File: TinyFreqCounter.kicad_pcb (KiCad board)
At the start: 2 copper layers, 99.1 x 82.5 mm, 30 parts, among them J1 Conn_01x20_Socket, J2 Conn_01x20_Socket, J3 Barrel_Jack_Switch, J4 Conn_01x06_Pin, J5 Conn_01x08_Pin, J6 Conn_01x06_Pin, J7 Conn_01x02_Pin, SW1 SW_SPDT, SW2 SW_SPST, U2 HM678127_SOJ32_Arranged, U3 PIC18F57Q43-IPT

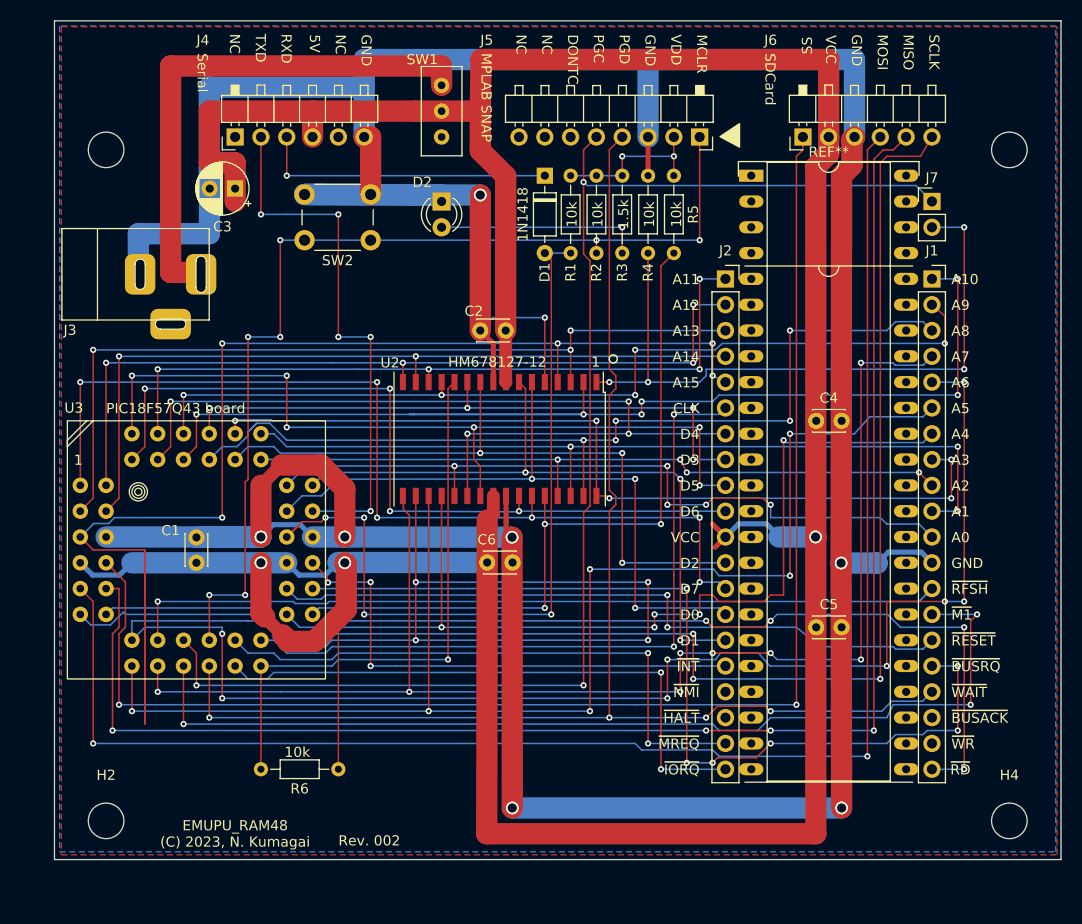
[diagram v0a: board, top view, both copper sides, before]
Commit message: Rev001: garber generated, and ordered to JLCPCB
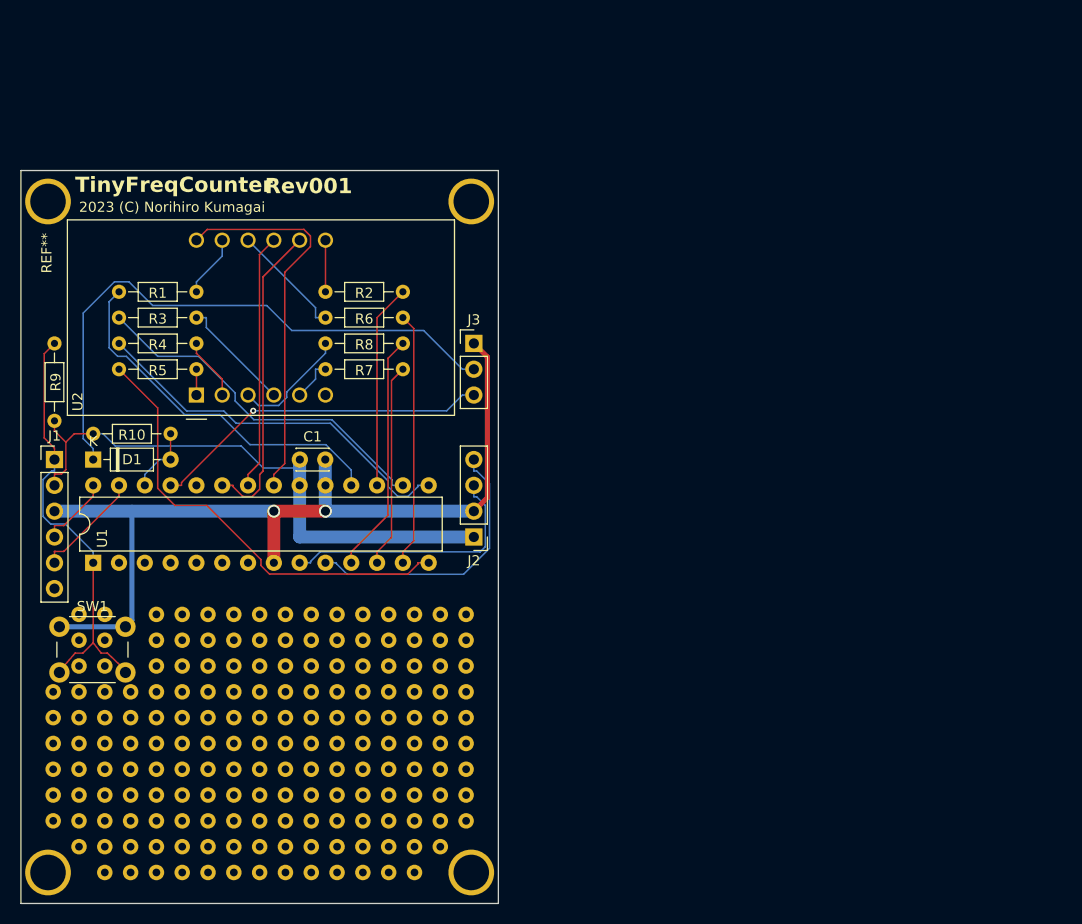
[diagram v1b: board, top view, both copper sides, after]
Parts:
- removed C2, C4, C5, C6: 0.1uF, Capacitor_THT:C_Disc_D3.0mm_W2.0mm_P2.50mm
- removed C3: 10uF, Capacitor_THT:CP_Radial_D5.0mm_P2.50mm
- removed D2: LED, LED_THT:LED_D3.0mm
- removed H2, H4, H5, H6: MountingHole, MountingHole:MountingHole_3.5mm
- removed J4, J6: Conn_01x06_Pin, 0-local:PinHeader_1x06_P2.54mm_Horizontal_NoFeet
- removed J5: Conn_01x08_Pin, 0-local:PinHeader_1x08_P2.54mm_Rev_Horizontal_Nofoot
- removed J7: Conn_01x02_Pin, Connector_PinHeader_2.54mm:PinHeader_1x02_P2.54mm_Vertical
- removed the REF** at (152.4, 73.7)
- removed SW2: SW_SPST, 0-local:SW_PUSH_6mm_H4.3mm
- removed U3: PIC18F57Q43-IPT, 0-local:Quad-2x6
- added R10: 10k, Resistor_THT:R_Axial_DIN0204_L3.6mm_D1.6mm_P7.62mm_Horizontal, F.Cu at (95.2, 99.1)
- added R7: 150, Resistor_THT:R_Axial_DIN0204_L3.6mm_D1.6mm_P7.62mm_Horizontal, F.Cu at (118.1, 92.7)
- added R8: 150, Resistor_THT:R_Axial_DIN0204_L3.6mm_D1.6mm_P7.62mm_Horizontal, F.Cu at (118.1, 90.2)
- added R9: 10k, Resistor_THT:R_Axial_DIN0204_L3.6mm_D1.6mm_P7.62mm_Horizontal, F.Cu at (83.8, 90.2)
- added REF**: Janome_16x10_half, 0-local:Janome_16x10_half, F.Cu at (83.7, 81.3)
- added U1: PIC18F27Q43-IP, Package_DIP:DIP-28_W7.62mm, F.Cu at (87.6, 111.8)
- J1: value Conn_01x20_Socket -> SNAP; footprint Connector_PinSocket_2.54mm:PinSocket_1x20_P2.54mm_Vertical -> Connector_PinHeader_2.54mm:PinHeader_1x06_P2.54mm_Vertical
- J2: value Conn_01x20_Socket -> CLKIO; footprint Connector_PinSocket_2.54mm:PinSocket_1x20_P2.54mm_Vertical -> Connector_PinHeader_2.54mm:PinHeader_1x04_P2.54mm_Vertical
- J3: value Barrel_Jack_Switch -> Serial; footprint 0-local:BARREL_JACK -> Connector_PinHeader_2.54mm:PinHeader_1x03_P2.54mm_Vertical
- R1, R2, R4, R5, R6: value 10k -> 150
- R3: value 1.5k -> 150
- SW1: value SW_SPDT -> SW_Push; footprint 0-local:PowerSW_for_SBC_series -> 0-local:SW_PUSH_6mm_H4.3mm
- U2: value HM678127_SOJ32_Arranged -> OSL-30561; footprint Package_SO:TSOP-II-32_21.0x10.2mm_P1.27mm -> 0-local:OSL-30561_no_courtyard
- moved J1 88.2 mm to (83.8, 101.6)
- moved SW1 63.2 mm to (84.3, 118.1), turned to 0 degrees
- moved R5 57.8 mm to (90.2, 92.7), turned to 0 degrees
- moved R4 52.8 mm to (90.2, 90.2), turned to 0 degrees
- moved D1 52.5 mm to (87.6, 101.6), turned to 0 degrees
- moved R3 51.5 mm to (90.2, 87.6), turned to 0 degrees
- moved R1 45.9 mm to (90.2, 85.1), turned to 0 degrees
- moved R6 44.9 mm to (118.1, 87.6)
- moved J2 35.5 mm to (125.1, 109.2), turned to 180 degrees
- moved J3 33.5 mm to (125.1, 90.2)
- moved U2 30.2 mm to (97.8, 95.2), turned to 90 degrees
- moved R2 22.2 mm to (118.1, 85.1), turned to 180 degrees
- moved C1 14.4 mm to (108.0, 101.6), turned to 0 degrees
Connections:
- D1 pad 2: Net-(D1-A) -> /TX1
- J1 pad 1: /A10 -> Net-(J1-Pin_1)
- J1 pad 2: /A9 -> VCC
- J1 pad 3: /A8 -> GND
- J1 pad 4: /A7 -> Net-(J1-Pin_4)
- J1 pad 5: /A6 -> Net-(J1-Pin_5)
- J1 pad 6: /A5 -> unconnected-(J1-Pin_6-Pad6)
- J2 pad 1: /A11 -> VCC
- J2 pad 2: /A12 -> GND
- J2 pad 3: /A13 -> Net-(J2-Pin_3)
- J2 pad 4: /A14 -> Net-(J2-Pin_4)
- J3 pad 1: Net-(SW1-C) -> GND
- J3 pad 2: GND -> Net-(D1-K)
- J3 pad 3: unconnected-(J3-Pad3) -> /RX1
- R1 pad 1: VCC -> Net-(U1-RC7)
- R1 pad 2: Net-(D1-A) -> Net-(U2-a)
- R2 pad 1: VCC -> Net-(U1-RC6)
- R2 pad 2: Net-(J5-Pin_1) -> Net-(U2-b)
- R3 pad 1: VCC -> Net-(U1-RC5)
- R3 pad 2: Net-(D2-A) -> Net-(U2-c)
- R4 pad 1: /A16 -> Net-(U1-RC4)
- R4 pad 2: GND -> Net-(U2-d)
- R5 pad 1: VCC -> Net-(U1-RC3)
- R5 pad 2: Net-(U2-~{OE}) -> Net-(U2-e)
- R6 pad 1: VCC -> Net-(U1-RC2)
- R6 pad 2: Net-(U2-~{WE}) -> Net-(U2-f)
- SW1 pad 1: unconnected-(SW1-A-Pad1) -> GND
- SW1 pad 2: VCC -> Net-(J1-Pin_1)
- U2 pad 1: /A16 -> Net-(U2-e)
- U2 pad 10: /D2 -> Net-(U2-f)
- U2 pad 11: /D3 -> Net-(U2-a)
- U2 pad 12: Net-(U2-~{WE}) -> Net-(U1-RB0)
- U2 pad 2: /A10 -> Net-(U2-d)
- U2 pad 3: /A13 -> Net-(U2-DP)
- U2 pad 4: /A15 -> Net-(U2-c)
- U2 pad 5: GND -> Net-(U2-g)
- U2 pad 6: /D0 -> unconnected-(U2-NC-Pad6)
- U2 pad 7: /D1 -> Net-(U2-b)
- U2 pad 8: VCC -> Net-(U1-RB2)
- U2 pad 9: GND -> Net-(U1-RB1)
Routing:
- net GND: track 399.6 -> 87.2 mm, vias 8 -> 2
- net VCC: track 358.6 -> 57.2 mm, vias 5 -> 0
- net /A6: track 222.0 -> 0.00 mm, vias 12 -> 0
- net Net-(J6-Pin_4): track 154.0 -> 0.00 mm, vias 2 -> 0
- net Net-(J6-Pin_5): track 150.7 -> 0.00 mm, vias 4 -> 0
- net Net-(J6-Pin_6): track 142.8 -> 0.00 mm, vias 3 -> 0
- net Net-(J6-Pin_1): track 137.8 -> 0.00 mm, vias 2 -> 0
- net /~{WAIT}: track 136.4 -> 0.00 mm, vias 4 -> 0
- net /A5: track 133.7 -> 0.00 mm, vias 6 -> 0
- net /TEST: track 133.2 -> 0.00 mm, vias 3 -> 0
- net /A7: track 132.0 -> 0.00 mm, vias 8 -> 0
- net /A15: track 129.7 -> 0.00 mm, vias 5 -> 0
- net /A10: track 116.2 -> 0.00 mm, vias 6 -> 0
- net /A4: track 115.2 -> 0.00 mm, vias 5 -> 0
- net Net-(J5-Pin_1): track 98.9 -> 0.00 mm, vias 7 -> 0
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- removed copper zone on B.Cu, net GND
- removed copper zone on F.Cu, net VCC
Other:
- board size 99.1 x 82.5 mm -> 47 x 72.1 mm
- board text added: "2023 (C) Norihiro Kumagai"
- board text added: "Rev001"
- board text added: "TinyFreqCounter"
- board text removed: "1"
- board text removed: "1.5k"
- board text removed: "10k"
- board text removed: "5V"
- board text removed: "A0"
- board text removed: "A1"
- board text removed: "A10"
- board text removed: "A11"
- board text removed: "A12"
- board text removed: "A13"
- board text removed: "A14"
- board text removed: "A15"
- board text removed: "A2"
- board text removed: "A3"
- board text removed: "A4"
- board text removed: "A5"
- board text removed: "A6"
- board text removed: "A7"
- board text removed: "A8"
- board text removed: "A9"
- board text removed: "CLK"
- board text removed: "D0"
- board text removed: "D1"
- board text removed: "D2"
- board text removed: "D3"
- board text removed: "D4"
- board text removed: "D5"
- board text removed: "D6"
- board text removed: "D7"
- board text removed: "DONTC"
- board text removed: "EMUPU_RAM48 (C) 2023, N. Kumagai"
- board text removed: "GND"
- board text removed: "HM678127-12"
- board text removed: "MCLR"
- board text removed: "MISO"
- board text removed: "MOSI"
- board text removed: "MPLAB SNAP"
- board text removed: "NC"
- board text removed: "PGC"
- board text removed: "PGD"
- board text removed: "PIC18F57Q43 board"
- board text removed: "RXD"
- board text removed: "Rev. 002"
- board text removed: "SCLK"
- board text removed: "SDCard"
- board text removed: "SS"
- board text removed: "Serial"
- board text removed: "TXD"
- board text removed: "VCC"
- board text removed: "VDD"
- board text removed: "~{BUSACK}"
- board text removed: "~{BUSRQ}"
- board text removed: "~{HALT}"
- board text removed: "~{INT}"
- board text removed: "~{IORQ}"
- board text removed: "~{M1}"
- board text removed: "~{MREQ}"
- board text removed: "~{NMI}"
- board text removed: "~{RD}"
- board text removed: "~{RESET}"
- board text removed: "~{RFSH}"
- board text removed: "~{WAIT}"
- board text removed: "~{WR}"
